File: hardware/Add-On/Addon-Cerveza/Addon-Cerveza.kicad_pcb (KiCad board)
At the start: 2 copper layers, 41.2 x 49.5 mm, 23 parts, among them J1 Conn_02x03_Odd_Even, SW2 On, SW7 RESET, U1 TMP102xxDRL, U2 CH32V003F4U6

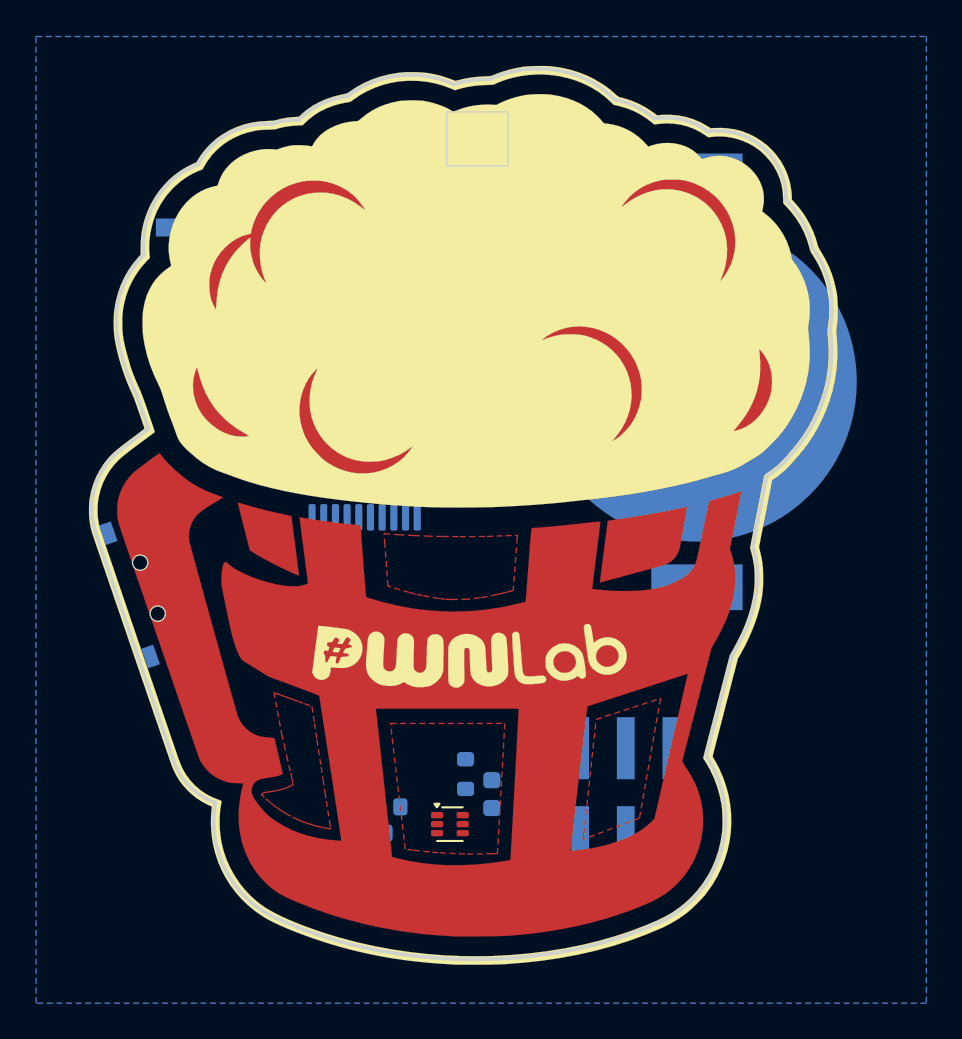
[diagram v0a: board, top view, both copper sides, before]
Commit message: feat(Hw):Init_Route_Add_On_Cerveza
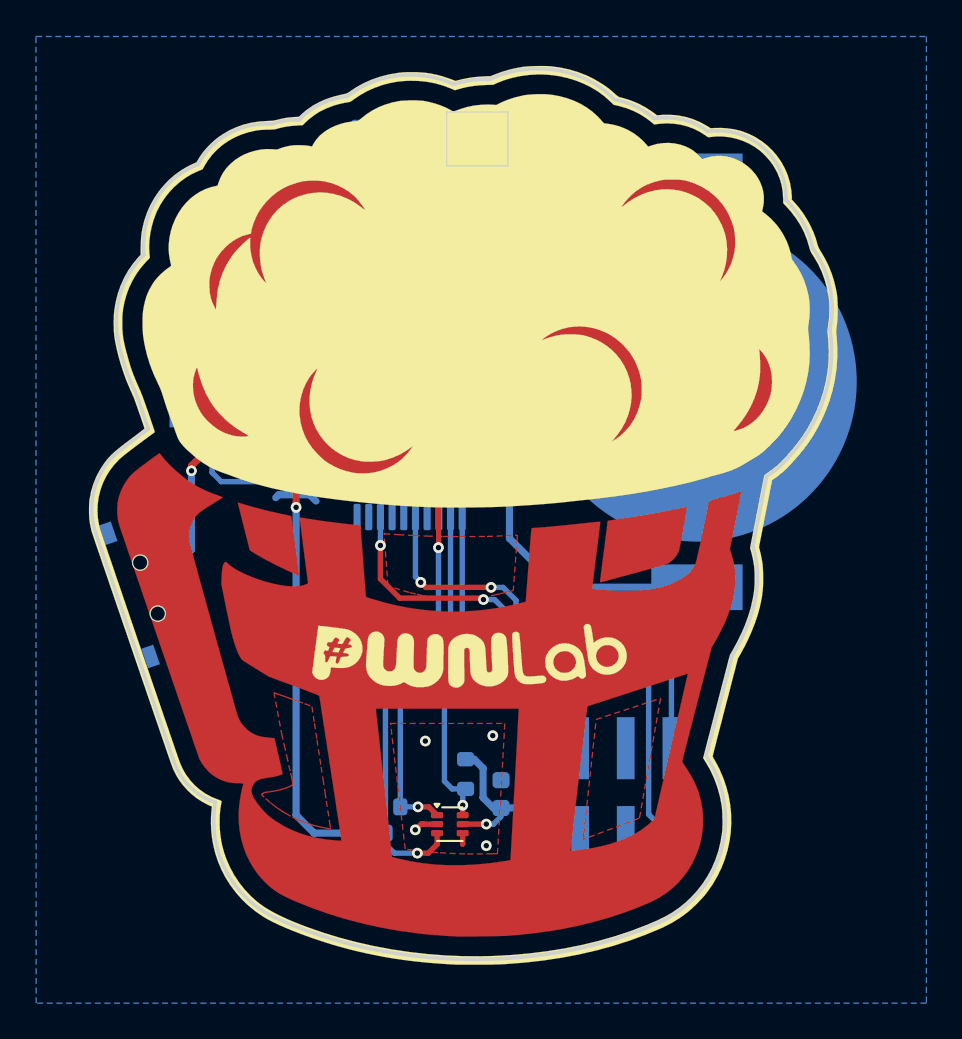
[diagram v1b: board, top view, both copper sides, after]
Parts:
- added ?: , , F.Cu at (88.4, 49.0)
- moved C8 5.69 mm to (82.9, 54.3)
- moved SW7 5.28 mm to (79.2, 54.3), turned to -90 degrees
- moved C7 2.50 mm to (92.4, 54.1)
- moved U2 2.50 mm to (90.1, 60.4)
- moved G*** 0.63 mm to (90.5, 70.0)
- moved C1 0.51 mm to (95.2, 78.7)
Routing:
- net +3V3: track 0.00 -> 124.1 mm, vias 0 -> 3
- net /NEOPIXELES: track 0.00 -> 39.0 mm
- net Net-(BT1--): track 0.00 -> 35.9 mm, vias 0 -> 4
- net /ALERT: track 0.00 -> 33.0 mm, vias 0 -> 3
- net /SWDIO: track 0.00 -> 31.4 mm, vias 0 -> 2
- net /SWCLK: track 0.00 -> 25.4 mm, vias 0 -> 2
- net /SCL: track 0.00 -> 20.3 mm, vias 0 -> 1
- net /SDA: track 0.00 -> 18.0 mm, vias 0 -> 1
- net /RST: track 0.00 -> 17.4 mm
- net GND: track 0.00 -> 12.7 mm, vias 0 -> 8
- net Net-(D11-DIN): track 0.00 -> 2.67 mm
